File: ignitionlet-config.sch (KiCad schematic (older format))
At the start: 23 parts, among them U1 IGNITION001-QFN, U5 MT25QL128ABB8E12-0AUT, U6 AT25PE80-SSHN-B

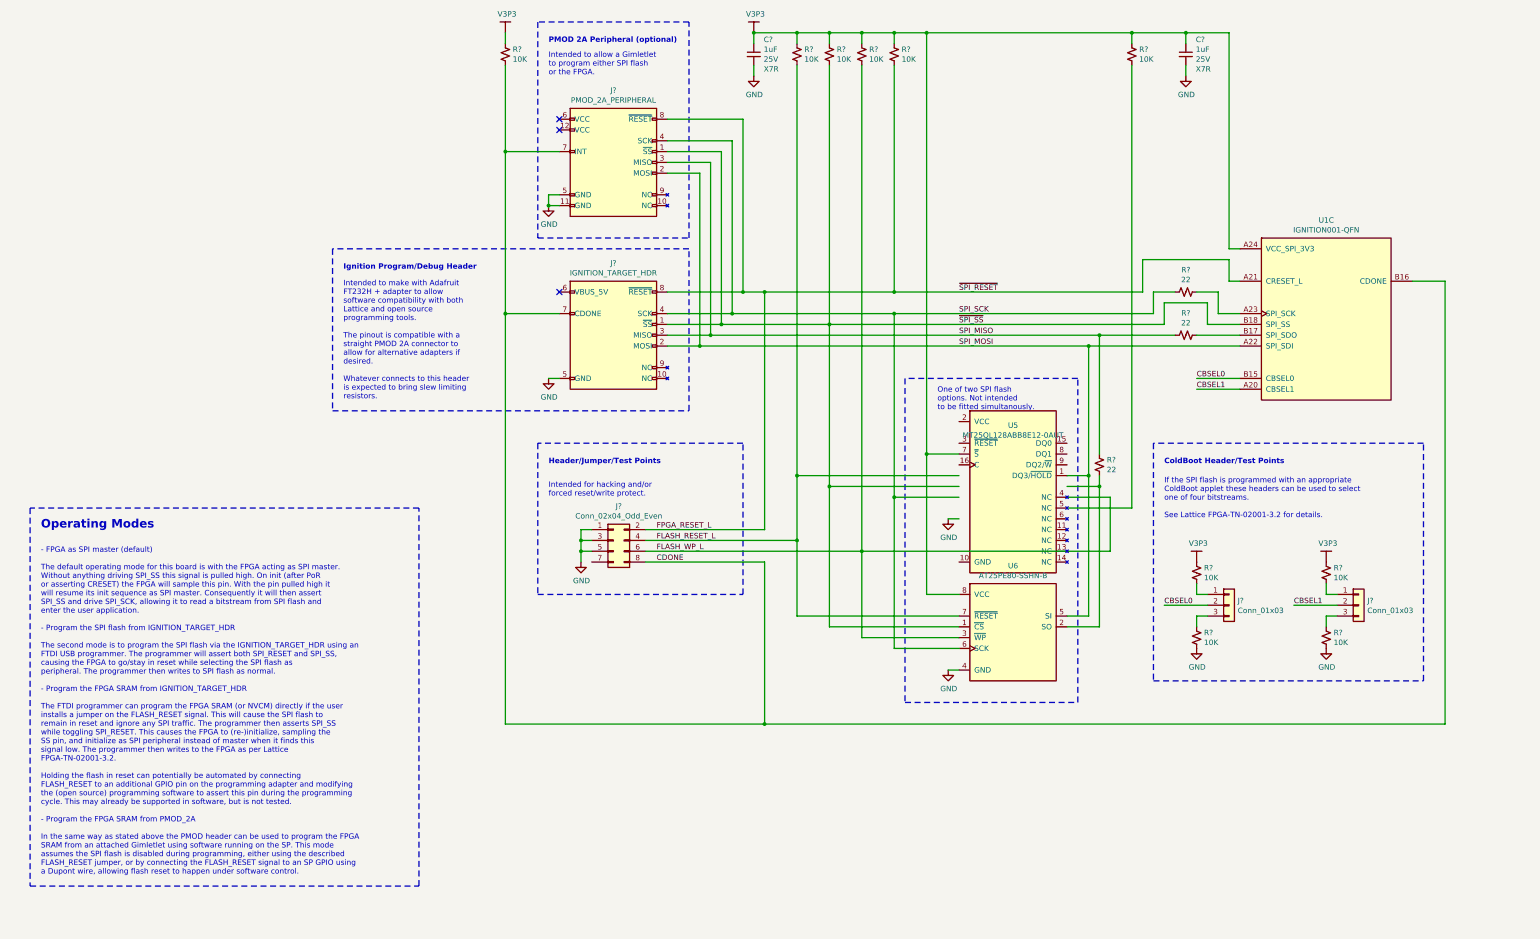
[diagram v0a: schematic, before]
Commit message: LED picked, fixed cap/resistor values, make RX hackable, improve readability
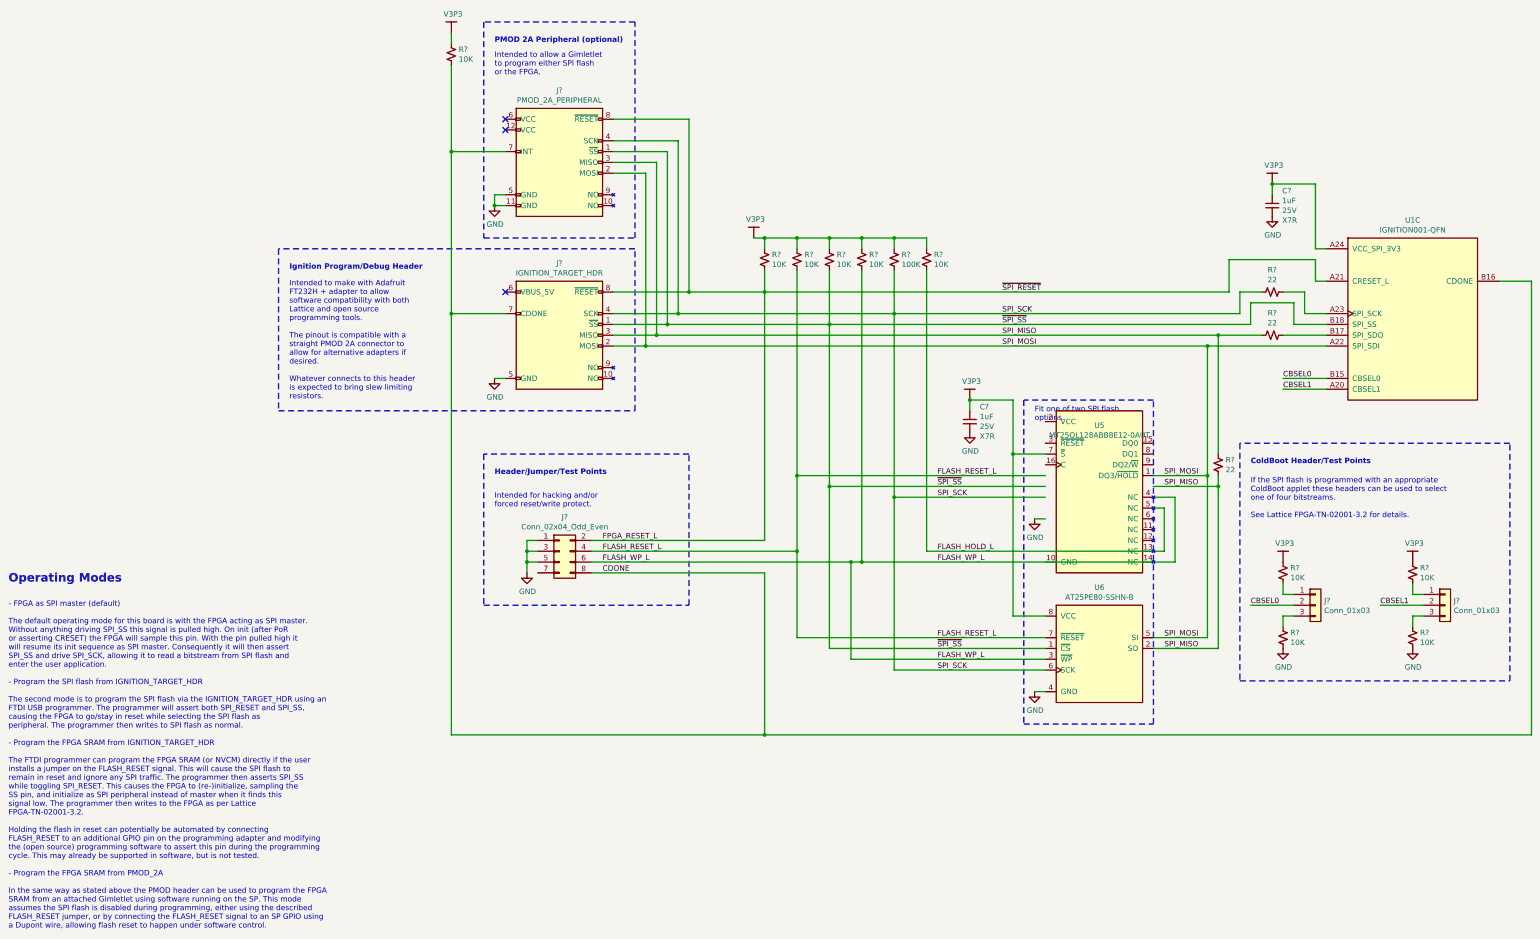
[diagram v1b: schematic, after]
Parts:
- added R?: 10K, Resistor_SMD:R_0603_1608Metric, symbol Device:R_Small_US
- R?: value 10K -> 100K
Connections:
- net labels added: FLASH_HOLD_L
- wire segments 135 -> 137
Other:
- note added: "Fit one of two SPI flash\noptions."
- note removed: "One of two SPI flash\noptions. Not intended\nto be fitted simultanously."
- moved on the sheet: C?, J?, R?, U1C, U5, U6
